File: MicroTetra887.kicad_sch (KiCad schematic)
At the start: 187 parts, among them J1 USB_B, J11 VGA DE15, J14 Conn_01x06, J15 Conn_01x06, J16 Conn_01x06, J8 DB9_Male, J9 DB9_Male, SW1 SW_Push, SW11 SW_Push, SW2 SW_Push, SW3 SW_Push, SW4 SW_Push, SW5 SW_Push, SW6 SW_Push, U1 PIC16F887-IP, Y1 Crystal

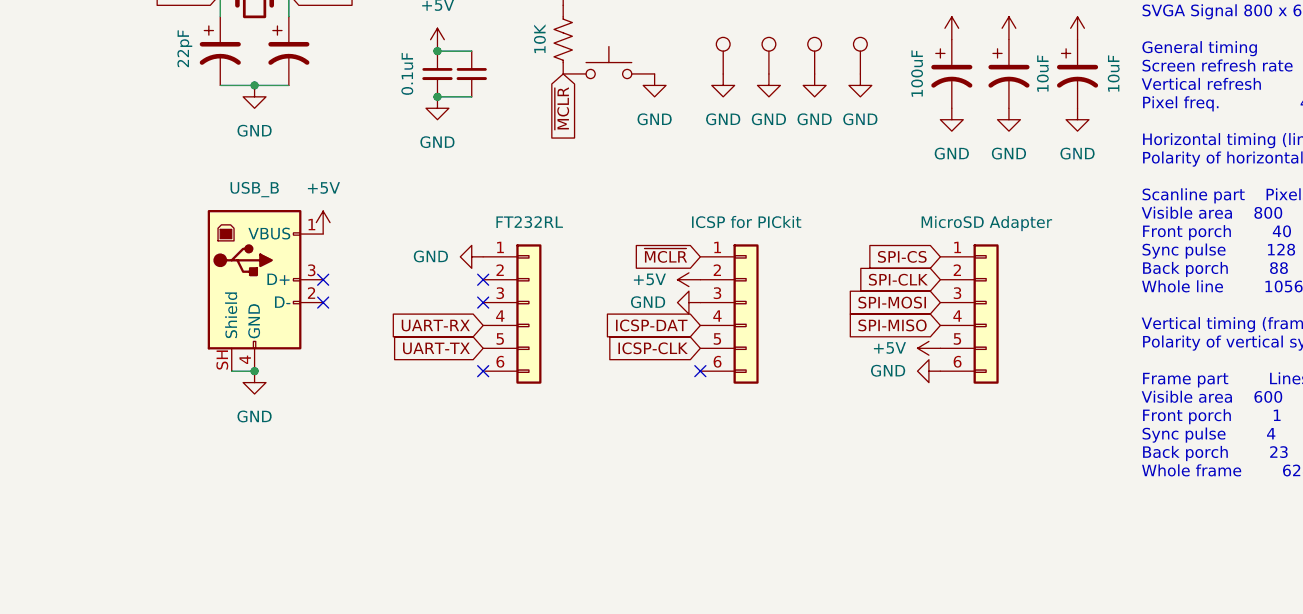
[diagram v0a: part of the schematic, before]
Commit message: Add files via upload
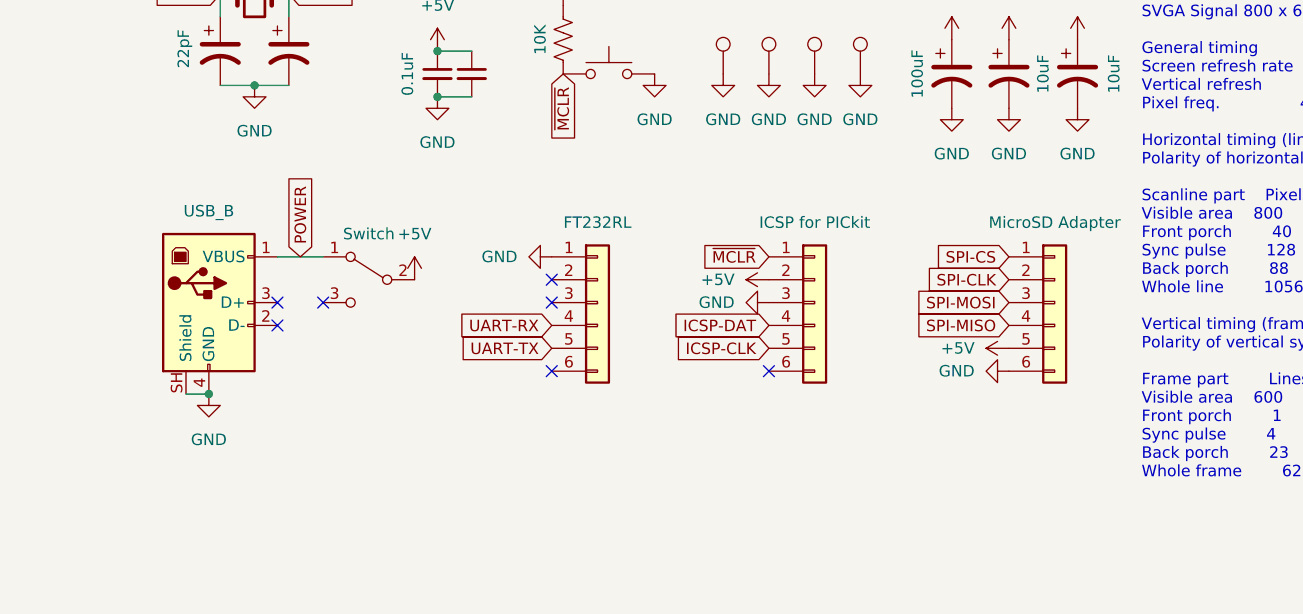
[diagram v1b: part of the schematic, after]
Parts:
- added SW7: SW_SPDT, Button_Switch_THT:SW_E-Switch_EG1224_SPDT_Angled, symbol Switch:SW_SPDT
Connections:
- net +5V: now also SW7.2 (B); no longer J1.1 (VBUS)
- new net POWER: J1.1 (VBUS), SW7.1 (A)
- no-connect marks 145 -> 146
